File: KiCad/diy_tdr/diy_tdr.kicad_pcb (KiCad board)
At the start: 2 copper layers, 25 parts, among them J1 DUT, J2 Scope, J3 Trig, U1 74HC14

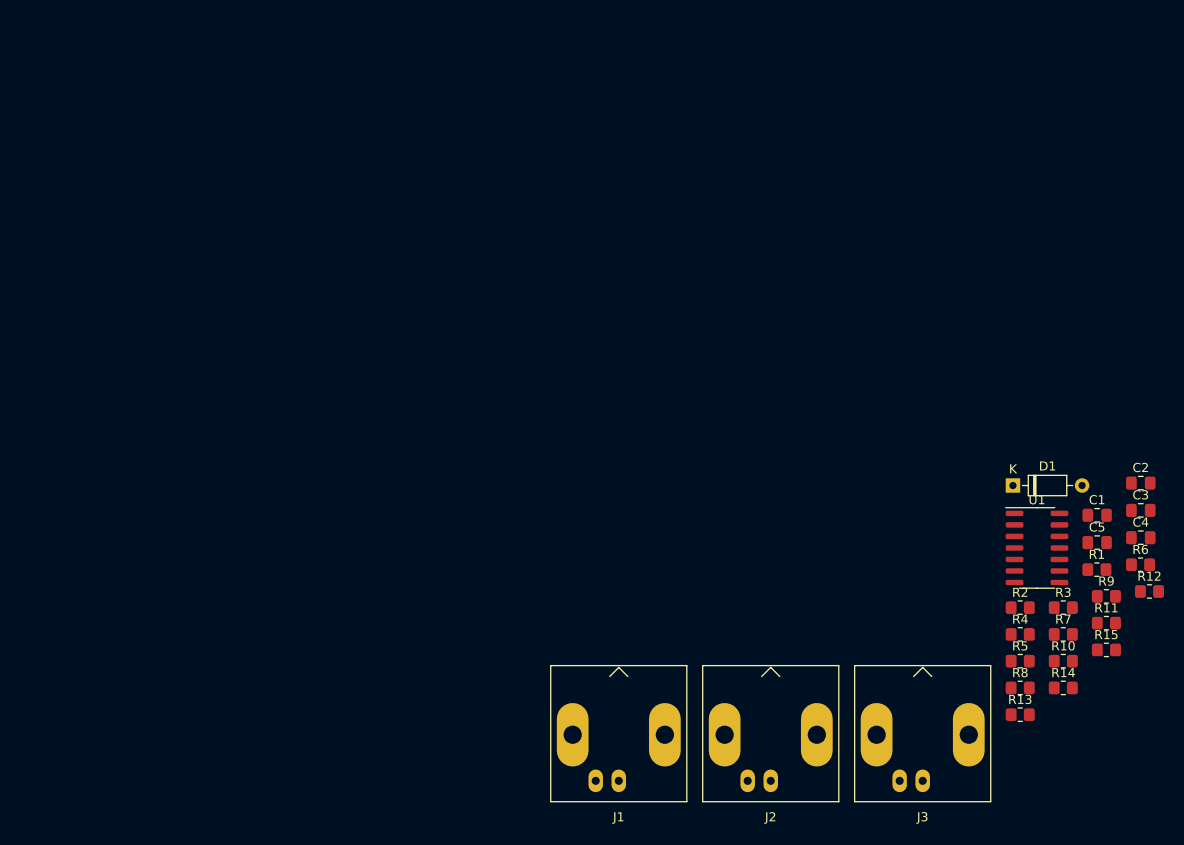
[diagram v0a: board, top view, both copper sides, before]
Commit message: finished layout
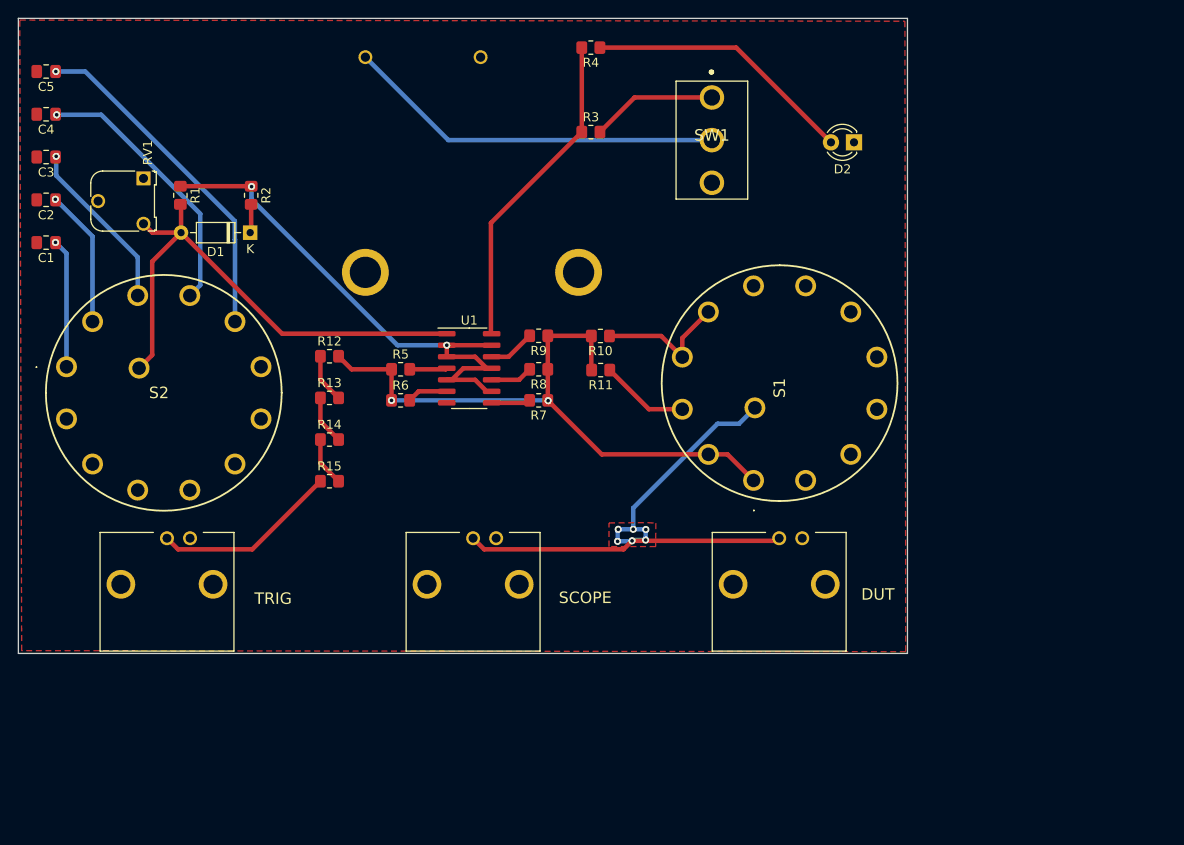
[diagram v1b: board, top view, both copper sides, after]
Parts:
- added BT1: Battery, SamacSys_Parts:2479, B.Cu at (65.0, 40.0)
- added D2: LED, LED_THT:LED_D3.0mm, F.Cu at (107.1, 25.7)
- added RV1: R_POT_TRIM_US, Potentiometer_THT:Potentiometer_Runtron_RM-065_Vertical, F.Cu at (28.8, 29.6)
- added S1: A10303RNCB, SamacSys_Parts:A10405RNCQE, F.Cu at (96.0, 62.9)
- added S2: A10303RNCB, SamacSys_Parts:A10405RNCQE, F.Cu at (20.3, 50.4)
- added SW1: SW_SPDT, SamacSys_Parts:M2012LL1W03, F.Cu at (91.4, 20.7)
- DUT: renamed from J1; footprint Connector_Coaxial:BNC_Amphenol_B6252HB-NPP3G-50_Horizontal -> SamacSys_Parts:731375003
- SCOPE: renamed from J2; footprint Connector_Coaxial:BNC_Amphenol_B6252HB-NPP3G-50_Horizontal -> SamacSys_Parts:731375003
- TRIG: renamed from J3; footprint Connector_Coaxial:BNC_Amphenol_B6252HB-NPP3G-50_Horizontal -> SamacSys_Parts:731375003
- moved C4 129.4 mm to (18.1, 22.6), turned to 180 degrees
- moved C5 127.0 mm to (18.1, 17.9), turned to 180 degrees
- moved C3 126.8 mm to (18.1, 27.3), turned to 180 degrees
- moved C2 124.6 mm to (18.1, 32.0), turned to 180 degrees
- moved C1 119.7 mm to (18.1, 36.7), turned to 180 degrees
- moved R1 109.1 mm to (32.9, 31.5), turned to 270 degrees
- moved R2 96.2 mm to (40.7, 31.5), turned to 270 degrees
- moved R12 94.0 mm to (49.3, 49.2)
- moved D1 88.6 mm to (40.6, 35.6), turned to 180 degrees
- moved R15 87.6 mm to (49.3, 63.0)
- moved TRIG 87.5 mm to (31.4, 69.3)
- moved R14 85.4 mm to (49.3, 58.4)
- moved R13 83.8 mm to (49.3, 53.8)
- moved R6 83.5 mm to (57.1, 54.1)
- moved R4 80.1 mm to (78.1, 15.2), turned to 180 degrees
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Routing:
- net Net-(R10-Pad2): track 0.00 -> 69.2 mm, vias 0 -> 2
- net Net-(J1-Pad1): track 0.00 -> 63.8 mm, vias 0 -> 6
- net Net-(R1-Pad1): track 0.00 -> 60.1 mm, vias 0 -> 2
- net Net-(D1-Pad2): track 0.00 -> 58.4 mm
- net Net-(BT1-Pad1): track 0.00 -> 42.0 mm
- net Net-(C5-Pad1): track 0.00 -> 37.6 mm, vias 0 -> 1
- net Net-(R3-Pad1): track 0.00 -> 35.7 mm
- net Net-(C4-Pad1): track 0.00 -> 29.8 mm, vias 0 -> 1
- net Net-(D2-Pad2): track 0.00 -> 29.8 mm
- net Net-(J3-Pad1): track 0.00 -> 20.5 mm
- net Net-(C3-Pad1): track 0.00 -> 19.1 mm, vias 0 -> 1
- net Net-(C2-Pad1): track 0.00 -> 15.2 mm, vias 0 -> 1
- net Net-(R10-Pad1): track 0.00 -> 15.2 mm
- net Net-(C1-Pad1): track 0.00 -> 14.2 mm, vias 0 -> 1
- net Net-(R3-Pad2): track 0.00 -> 13.9 mm
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- added copper zone on F.Cu, net GND
- added copper zone on F.Cu, net Net-(J1-Pad1)
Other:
- board outline added: 98 x 70 mm
